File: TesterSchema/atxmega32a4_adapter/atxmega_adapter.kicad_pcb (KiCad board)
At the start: 2 copper layers, 55 x 20 mm, 23 parts, among them IC1 ATXMEGA32A4-M, P1 DIL40, Q1 BC817-40, Q2 BC817-40, Q3 BC817-40, U1 APE8865N-33-HF-3

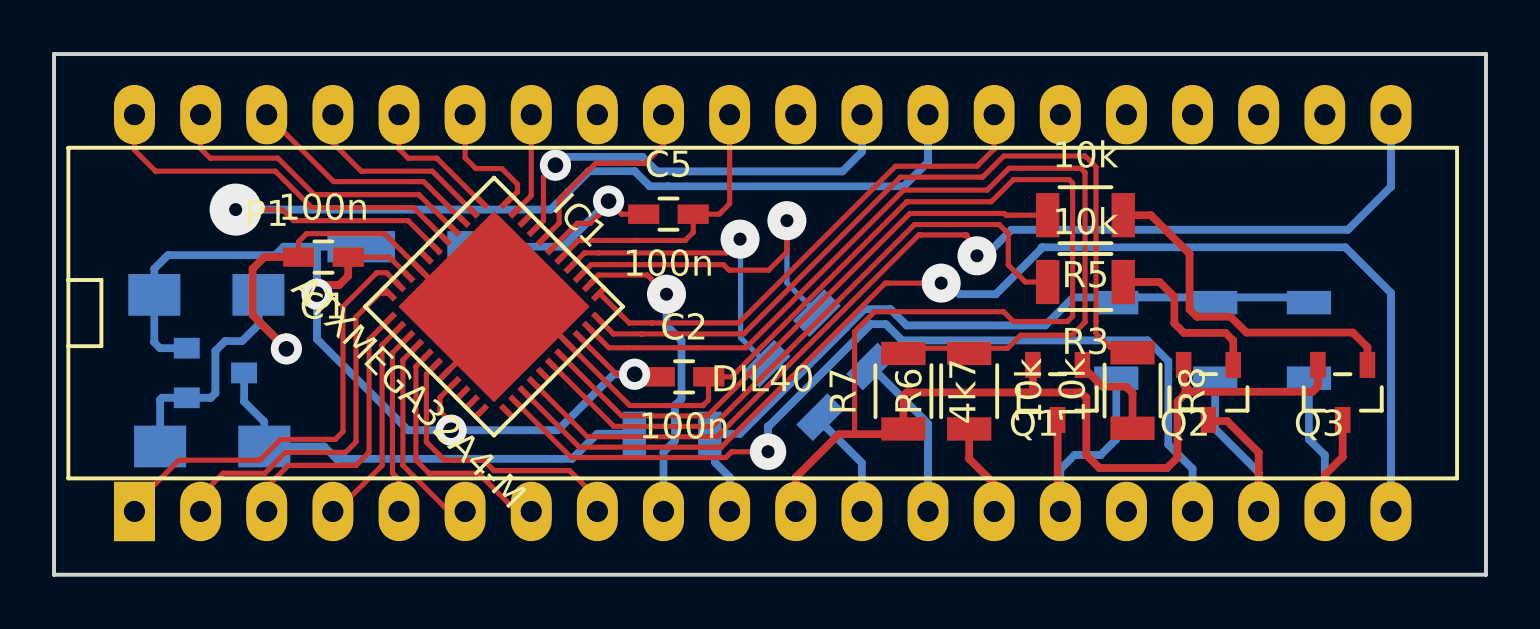
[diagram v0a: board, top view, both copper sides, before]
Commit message: poprawki płytki
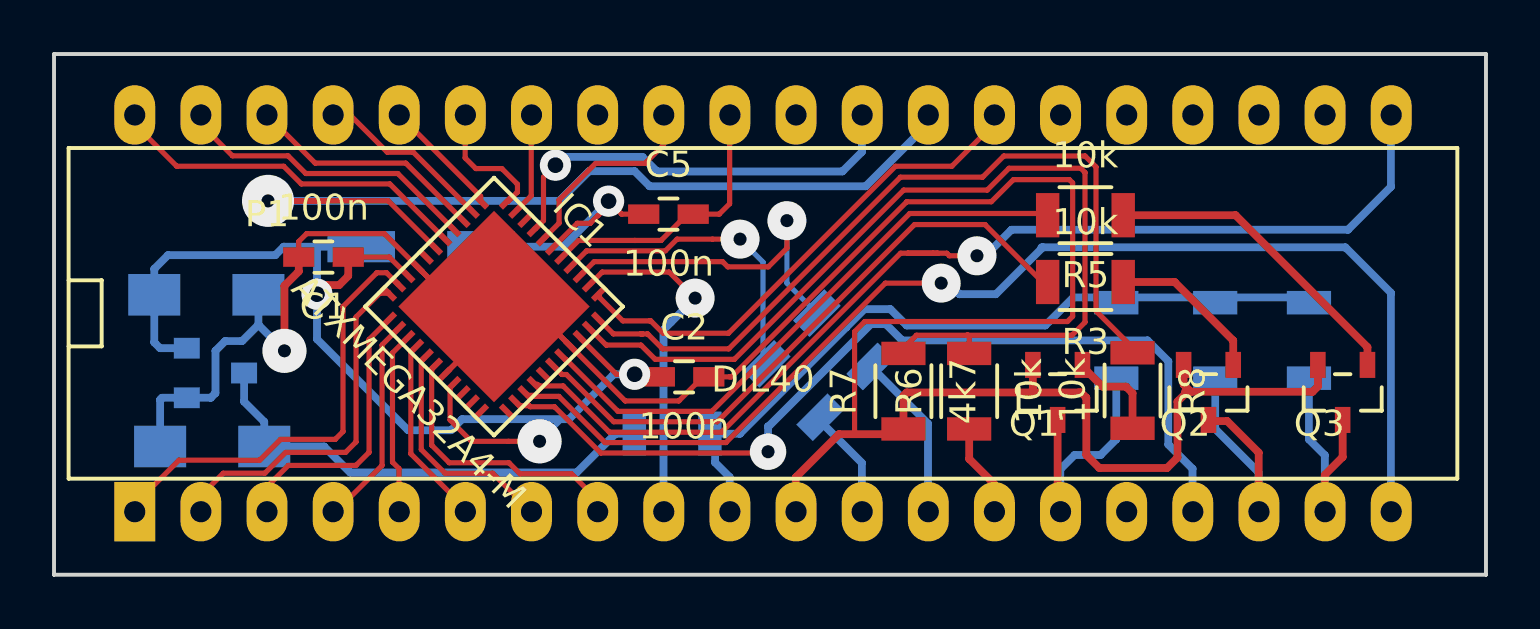
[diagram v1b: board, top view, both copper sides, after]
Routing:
- net +3.3V: track 41.2 -> 45.7 mm
- net GND: track 120.4 -> 116.8 mm
- net /SW1: track 38.2 -> 36.8 mm
- net /DB5: track 8.37 -> 7.05 mm
- net Net-(Q3-Pad1): track 13.2 -> 11.9 mm
- net /DB7: track 11.5 -> 10.3 mm
- net Net-(IC1-Pad32): track 35.4 -> 36.5 mm
- net /RESET: track 12.5 -> 13.4 mm
- net Net-(IC1-Pad28): track 24.6 -> 23.7 mm
- net /ADC_I: track 5.39 -> 4.73 mm
- net /E: track 7.48 -> 6.85 mm
- net Net-(Q2-Pad1): track 6.45 -> 5.85 mm
- net /ADC_U: track 14.6 -> 14.1 mm
- net /DB6: track 9.38 -> 8.83 mm
- net /RS: track 12.3 -> 11.7 mm
